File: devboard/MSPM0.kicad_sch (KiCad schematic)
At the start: 64 parts, among them J1 Conn_01x02, J2 Conn_01x03_Pin, J3 SWD, J5 Conn_01x03_Pin, SW1 SW_Push, SW2 SW_Push, SW3 SW_Push, SW4 SW, U1 AP2112K-3.3, Y1 40MHz

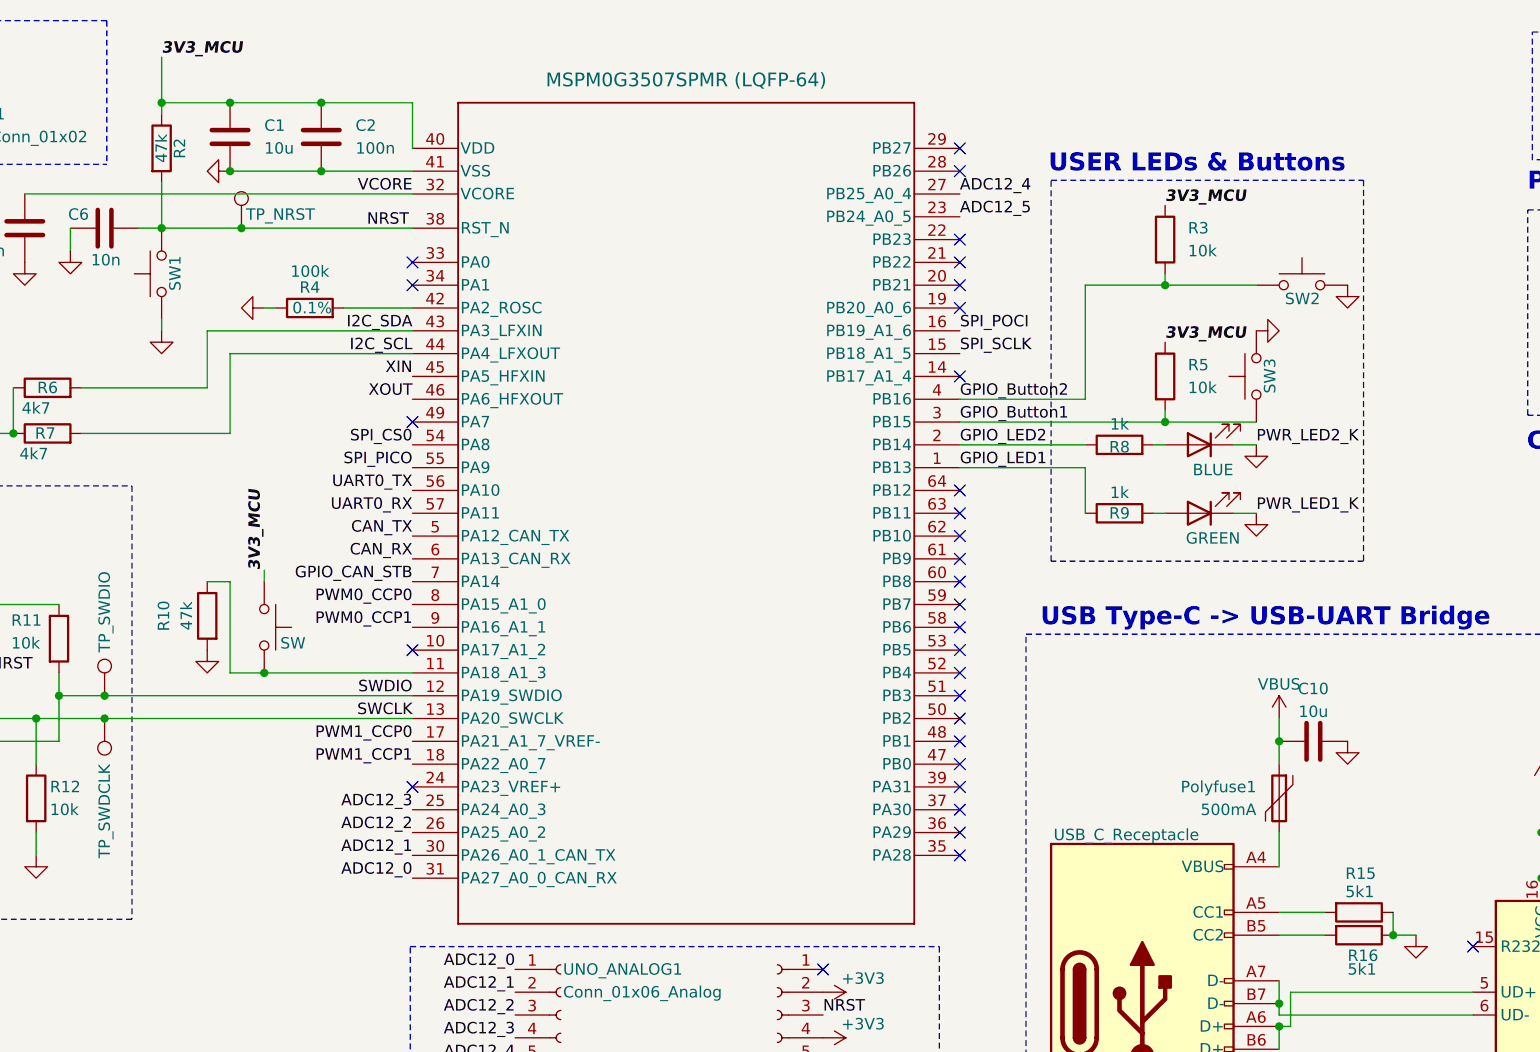
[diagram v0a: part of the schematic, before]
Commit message: started layout, but <bruhh> i forgot i couldnt edit layout of mcu
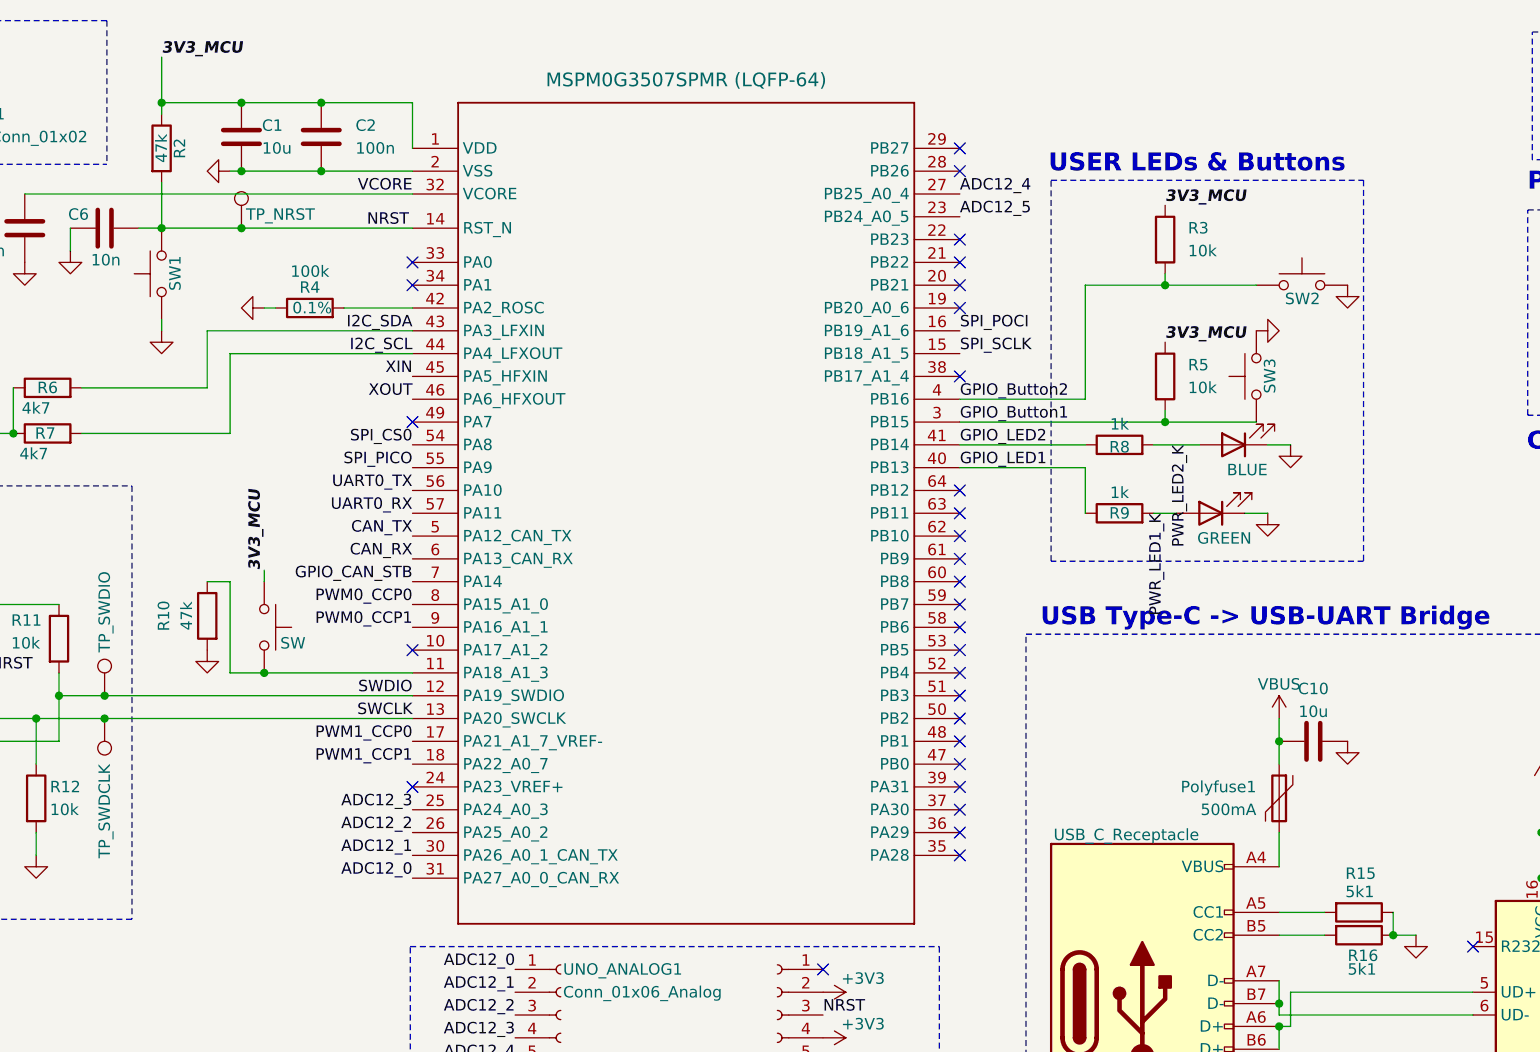
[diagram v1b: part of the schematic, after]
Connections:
- net 3V3_MCU: now also MCU1.1 (VDD); no longer MCU1.40 (VDD)
- net GND: now also MCU1.2 (VSS); no longer MCU1.41 (VSS)
- net GPIO_LED1: now also MCU1.40 (PB13); no longer MCU1.1 (PB13)
- net GPIO_LED2: now also MCU1.41 (PB14); no longer MCU1.2 (PB14)
- net NRST: now also MCU1.14 (RST_N); no longer MCU1.38 (RST_N)
- net PWR_LED1_K: now reaches D3.2 (A), R9.2
- net PWR_LED2_K: now reaches D2.2 (A), R8.2
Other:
- moved on the sheet: C1
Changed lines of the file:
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@@
 	)
 	(junction
-		(at 99.06 21.59)
-		(diameter 0)
-		(color 0 0 0 0)
-	)
-	(junction
 		(at 85.09 90.17)
 		(diameter 0)
@@
 	)
 	(junction
-		(at 99.06 29.21)
+		(at 228.6 114.3)
 		(diameter 0)
 		(color 0 0 0 0)
 	)
 	(junction
-		(at 228.6 114.3)
+		(at 255.27 41.91)
 		(diameter 0)
 		(color 0 0 0 0)
 	)
 	(junction
-		(at 255.27 41.91)
+		(at 100.33 29.21)
 		(diameter 0)
 		(color 0 0 0 0)
@@
 	)
 	(junction
+		(at 100.33 21.59)
+		(diameter 0)
+		(color 0 0 0 0)
+	)
+	(junction
 		(at 215.9 124.46)
 		(diameter 0)
@@
 	(wire
 		(pts
+			(xy 100.33 29.21) (xy 109.22 29.21)
+		)
+		(stroke
+			(width 0)
+			(type default)
+		)
+	)
+	(wire
+		(pts
 			(xy 215.9 121.92) (xy 215.9 123.19)
 		)
@@
 	(wire
 		(pts
+			(xy 100.33 21.59) (xy 109.22 21.59)
+		)
+		(stroke
+			(width 0)
+			(type default)
+		)
+	)
+	(wire
+		(pts
 			(xy 72.39 58.42) (xy 74.93 58.42)
 		)
@@
 	(wire
 		(pts
-			(xy 91.44 21.59) (xy 99.06 21.59)
+			(xy 91.44 21.59) (xy 100.33 21.59)
 		)
 		(stroke
@@
 	(wire
 		(pts
-			(xy 203.2 67.31) (xy 201.93 67.31)
+			(xy 201.93 67.31) (xy 204.47 67.31)
 		)
 		(stroke
@@
 	(wire
 		(pts
-			(xy 203.2 59.69) (xy 201.93 59.69)
+			(xy 207.01 59.69) (xy 201.93 59.69)
 		)
 		(stroke
@@
 	(wire
 		(pts
-			(xy 99.06 29.21) (xy 109.22 29.21)
+			(xy 99.06 29.21) (xy 100.33 29.21)
 		)
 		(stroke
@@
 	(wire
 		(pts
-			(xy 210.82 67.31) (xy 213.36 67.31)
+			(xy 212.09 67.31) (xy 214.63 67.31)
 		)
 		(stroke
@@
 	(wire
 		(pts
-			(xy 99.06 21.59) (xy 109.22 21.59)
-		)
-		(stroke
-			(width 0)
-			(type default)
-		)
-	)
-	(wire
-		(pts
 			(xy 203.2 41.91) (xy 194.31 41.91)
 		)
@@
 	(wire
 		(pts
-			(xy 210.82 59.69) (xy 213.36 59.69)
+			(xy 214.63 59.69) (xy 217.17 59.69)
 		)
 		(stroke
@@
 	)
 	(label "PWR_LED1_K"
-		(at 213.36 67.31 0)
+		(at 203.2 67.31 270)
 		(effects
 			(font
 				(size 1.27 1.27)
 			)
-			(justify left bottom)
+			(justify right bottom)
 		)
 	)
@@
 	)
 	(label "PWR_LED2_K"
-		(at 213.36 59.69 0)
+		(at 205.74 59.69 270)
 		(effects
 			(font
 				(size 1.27 1.27)
 			)
-			(justify left bottom)
+			(justify right bottom)
 		)
 	)
@@
 	(symbol
 		(lib_id "Device:LED")
-		(at 207.01 67.31 180)
+		(at 208.28 67.31 180)
 		(unit 1)
 		(body_style 1)
@@
 		(dnp no)
 		(property "Reference" "D3"
-			(at 208.5975 59.69 0)
+			(at 209.8675 59.69 0)
 			(hide yes)
 			(show_name no)
@@
 		)
 		(property "Value" "GREEN"
-			(at 208.534 70.104 0)
+			(at 209.804 70.104 0)
 			(show_name no)
 			(do_not_autoplace no)
@@
 		)
 		(property "Footprint" "LED_SMD:LED_0603_1608Metric"
-			(at 207.01 67.31 0)
+			(at 208.28 67.31 0)
 			(hide yes)
 			(show_name no)
@@
 		)
 		(property "Datasheet" ""
-			(at 207.01 67.31 0)
+			(at 208.28 67.31 0)
 			(hide yes)
 			(show_name no)
@@
 		)
 		(property "Description" "Light emitting diode"
-			(at 207.01 67.31 0)
+			(at 208.28 67.31 0)
 			(hide yes)
 			(show_name no)
@@
 		)
 		(property "Sim.Pins" "1=K 2=A"
-			(at 207.01 67.31 0)
+			(at 208.28 67.31 0)
 			(hide yes)
 			(show_name no)
@@
 	(symbol
 		(lib_id "Device:C")
-		(at 99.06 25.4 0)
+		(at 100.33 25.4 0)
 		(unit 1)
 		(body_style 1)
@@
 		(in_pos_files yes)
 		(dnp no)
-		(fields_autoplaced yes)
 		(property "Reference" "C1"
-			(at 102.87 24.1299 0)
+			(at 102.616 24.13 0)
 			(show_name no)
 			(do_not_autoplace no)
@@
 		)
 		(property "Value" "10u"
-			(at 102.87 26.6699 0)
+			(at 102.616 26.67 0)
 			(show_name no)
 			(do_not_autoplace no)
@@
 		)
 		(property "Footprint" "Capacitor_SMD:C_0603_1608Metric"
-			(at 100.0252 29.21 0)
+			(at 101.2952 29.21 0)
 			(hide yes)
 			(show_name no)
@@
 		)
 		(property "Datasheet" ""
-			(at 99.06 25.4 0)
+			(at 100.33 25.4 0)
 			(hide yes)
 			(show_name no)
@@
 		)
 		(property "Description" "Unpolarized capacitor"
-			(at 99.06 25.4 0)
+			(at 100.33 25.4 0)
 			(hide yes)
 			(show_name no)
@@
 	(symbol
 		(lib_id "power:GND")
-		(at 213.36 59.69 0)
+		(at 217.17 59.69 0)
 		(unit 1)
 		(body_style 1)
@@
 		(fields_autoplaced yes)
 		(property "Reference" "#PWR021"
-			(at 213.36 66.04 0)
+			(at 217.17 66.04 0)
 			(hide yes)
 			(show_name no)
@@
 		)
 		(property "Value" "GND"
-			(at 213.36 64.77 0)
+			(at 217.17 64.77 0)
 			(hide yes)
 			(show_name no)
@@
 		)
 		(property "Footprint" ""
-			(at 213.36 59.69 0)
+			(at 217.17 59.69 0)
 			(hide yes)
 			(show_name no)
@@
 		)
 		(property "Datasheet" ""
-			(at 213.36 59.69 0)
+			(at 217.17 59.69 0)
 			(hide yes)
 			(show_name no)
@@
 		)
 		(property "Description" "Power symbol creates a global label with name \"GND\" , ground"
-			(at 213.36 59.69 0)
+			(at 217.17 59.69 0)
 			(hide yes)
 			(show_name no)
@@
 	(symbol
 		(lib_id "power:GND")
-		(at 213.36 67.31 0)
+		(at 214.63 67.31 0)
 		(unit 1)
 		(body_style 1)
@@
 		(fields_autoplaced yes)
 		(property "Reference" "#PWR022"
-			(at 213.36 73.66 0)
+			(at 214.63 73.66 0)
 			(hide yes)
 			(show_name no)
@@
 		)
 		(property "Value" "GND"
-			(at 213.36 72.39 0)
+			(at 214.63 72.39 0)
 			(hide yes)
 			(show_name no)
@@
 		)
 		(property "Footprint" ""
-			(at 213.36 67.31 0)
+			(at 214.63 67.31 0)
 			(hide yes)
 			(show_name no)
@@
 		)
 		(property "Datasheet" ""
-			(at 213.36 67.31 0)
+			(at 214.63 67.31 0)
 			(hide yes)
 			(show_name no)
@@
 		)
 		(property "Description" "Power symbol creates a global label with name \"GND\" , ground"
-			(at 213.36 67.31 0)
+			(at 214.63 67.31 0)
 			(hide yes)
 			(show_name no)
@@
 	(symbol
 		(lib_id "Device:LED")
-		(at 207.01 59.69 180)
+		(at 210.82 59.69 180)
 		(unit 1)
 		(body_style 1)
@@
 		(dnp no)
 		(property "Reference" "D2"
-			(at 208.5975 52.07 0)
+			(at 212.4075 52.07 0)
 			(hide yes)
 			(show_name no)
@@
 		)
 		(property "Value" "BLUE"
-			(at 208.534 62.484 0)
+			(at 212.344 62.484 0)
 			(show_name no)
 			(do_not_autoplace no)
@@
 		)
 		(property "Footprint" "LED_SMD:LED_0603_1608Metric"
-			(at 207.01 59.69 0)
+			(at 210.82 59.69 0)
 			(hide yes)
 			(show_name no)
@@
 		)
 		(property "Datasheet" ""
-			(at 207.01 59.69 0)
+			(at 210.82 59.69 0)
 			(hide yes)
 			(show_name no)
@@
 		)
 		(property "Description" "Light emitting diode"
-			(at 207.01 59.69 0)
+			(at 210.82 59.69 0)
 			(hide yes)
 			(show_name no)
@@
 		)
 		(property "Sim.Pins" "1=K 2=A"
-			(at 207.01 59.69 0)
+			(at 210.82 59.69 0)
 			(hide yes)
 			(show_name no)
